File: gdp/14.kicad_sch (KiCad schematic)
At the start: 0 parts

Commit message: Adds Sheet 12
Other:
- company: (none) -> Oddbit Retro
- title: (none) -> PARTNER GDP: CLOCK GEN
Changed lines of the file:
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@@
 	(generator_version "8.0")
 	(paper "A4")
+	(title_block
+		(title "PARTNER GDP: CLOCK GEN")
+		(company "Oddbit Retro")
+		(comment 1 "NARISAL: MIHA GRČAR")
+	)
 )

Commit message: Adds Sheet 14 (WIP)
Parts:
- added CK62: U22, symbol Device:C_Small
- added CK63: 10P, symbol Device:C_Small
- added IC61: 74LS163, symbol 74xx:74LS163
- added IC65, U7: 74LS74, symbol 74xx:74LS74
- added IC72, U13: 74LS04, symbol 74xx:74LS04
- added O1: Crystal, symbol Device:Crystal
- added R28, R51: 1K0, symbol Device:R
- added R50, R54: 470R, symbol Device:R
- added U10, U14, U15, U16, U17, U8, U9: 74LS00, symbol 74xx:74LS00
- added U11: 74LS123, symbol 74xx:74LS123
- added U12: 74LS14, symbol 74xx:74LS14
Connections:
- new net: IC72.2, IC72.3, O1.2, R54.2
- new net: IC61.2 (CP), IC72.4, IC72.9, R28.2
- new net: CK62.2, IC72.1, R54.1
- new net: CK62.1, IC72.12, R50.2
- new net: CK63.1, IC72.13, O1.1, R50.1
- new net: IC61.1 (~{MR}), IC61.10 (CET)
- new net +5V: IC61.16 (VCC), IC61.9 (~{PE}), IC65.10 (~{S}), IC65.13 (~{R}), R51.1
- new net EOC: IC61.15 (TC)
- new net GNDD: CK63.2, IC61.3 (D0), IC61.4 (D1), IC61.5 (D2), IC61.6 (D3), IC61.8 (GND), R28.1
- new net MUX1: IC65.8 (~{Q})
- new net QA: IC61.13 (Q1), IC65.11 (C)
- new net QB: IC61.12 (Q2)
- new net QC: IC61.11 (Q3), IC65.12 (D)
- no-connect marks 0 -> 2

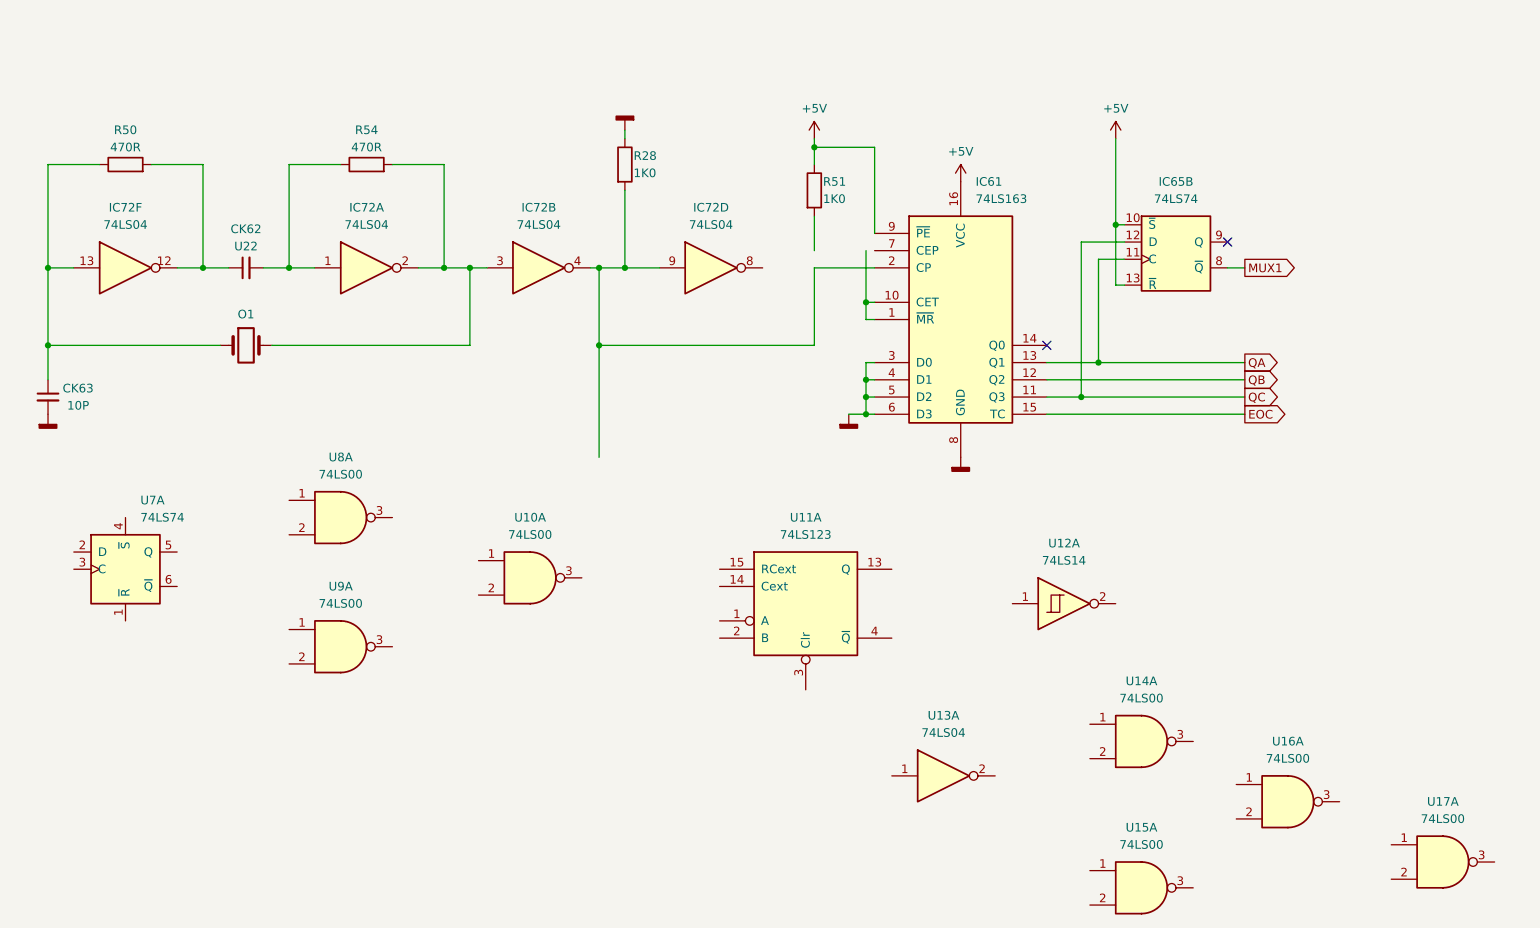
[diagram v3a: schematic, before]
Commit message: Adds Sheet 14
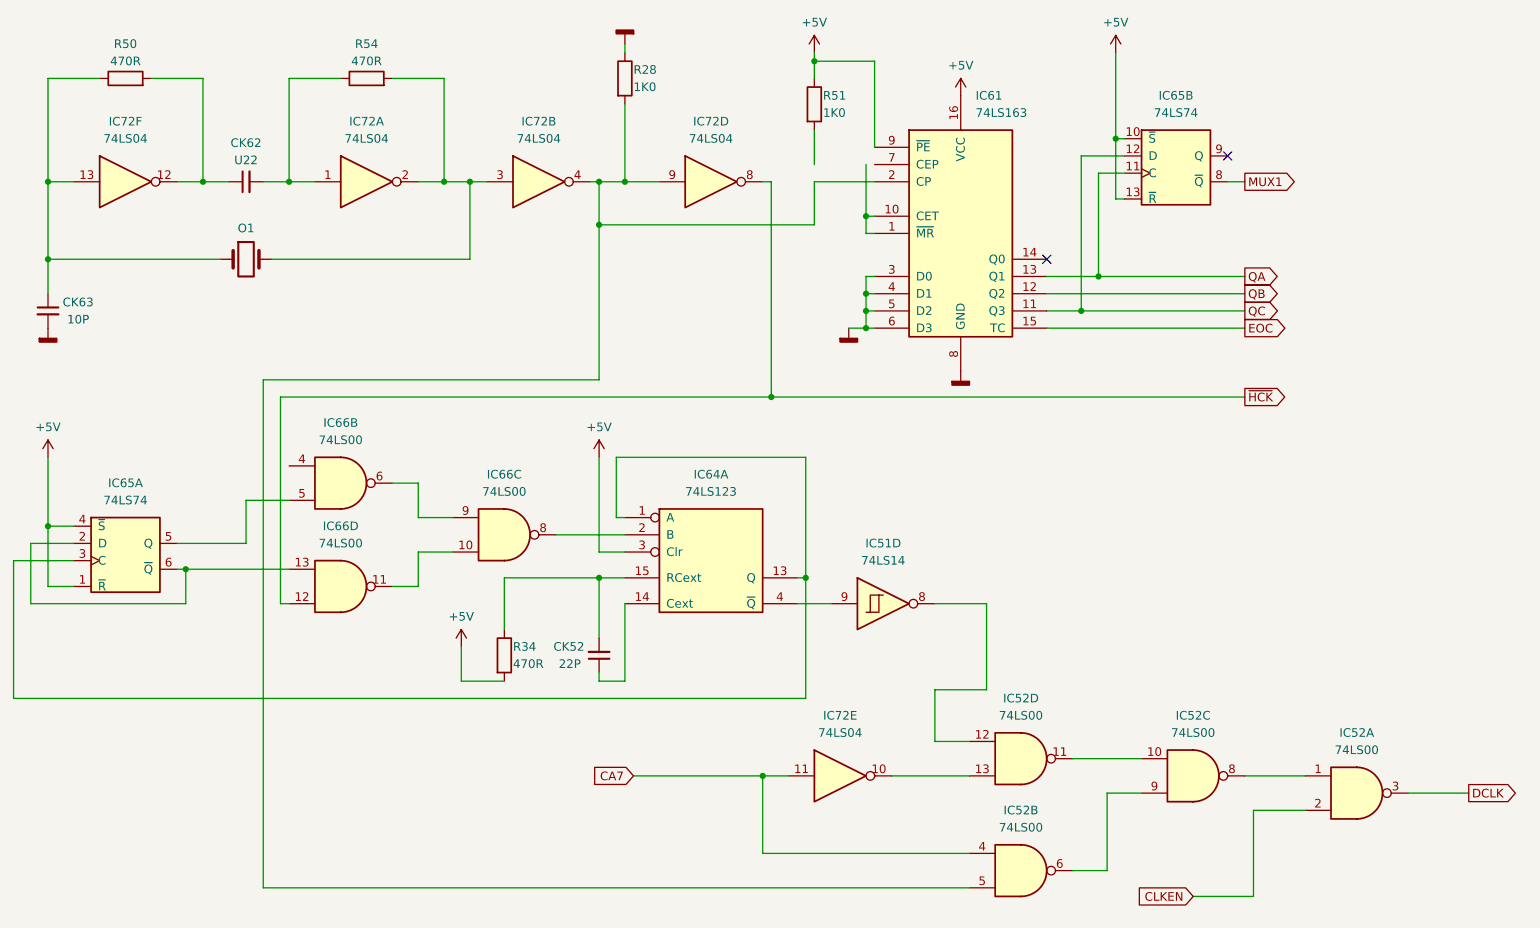
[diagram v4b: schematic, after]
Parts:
- added CK52: 22P, symbol Device:C_Small
- added R34: 470R, symbol Device:R
- renumbered U12 to IC51, U14 to IC52, U17 to IC52, U15 to IC52, U16 to IC52, U11 to IC64, U7 to IC65, U8 to IC66, U9 to IC66, U10 to IC66, U13 to IC72
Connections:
- net +5V: now also IC64.3 (Clr), IC65.1 (~{R}), IC65.4 (~{S}), R34.2
- net at IC61.2 (CP), IC72.4, IC72.9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: now also IC52.5
- net at IC52.1: now also IC52.8
- net CLKEN: now reaches IC52.2
- net DCLK: now reaches IC52.3
- net at IC65.2 (D): now also IC65.6 (~{Q}), IC66.13
- net at IC65.3 (C): now also IC64.1 (A), IC64.13 (Q)
- net at IC65.5 (Q): now also IC66.5
- net ~{HCK}: now reaches IC72.8
- net ~{HCK}: now also IC66.12
- net at IC64.14 (Cext): now also CK52.1
- net at IC64.15 (RCext): now also CK52.2, R34.1
- net at IC64.2 (B): now also IC66.8
- net at IC64.4 (~{Q}): now also IC51.9
- new net: IC52.10, IC52.11
- new net: IC51.8, IC52.12
- new net: IC52.13, IC72.10
- new net: IC52.6, IC52.9
- new net: IC66.6, IC66.9
- new net: IC66.10, IC66.11
- new net CA7: IC52.4, IC72.11
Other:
- moved on the sheet: CK62, CK63, IC51D, IC52A, IC52B, IC52C, IC52D, IC61, IC64A, IC65A, IC65B, IC66B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
